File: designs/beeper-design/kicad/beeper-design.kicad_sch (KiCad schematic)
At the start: 0 parts

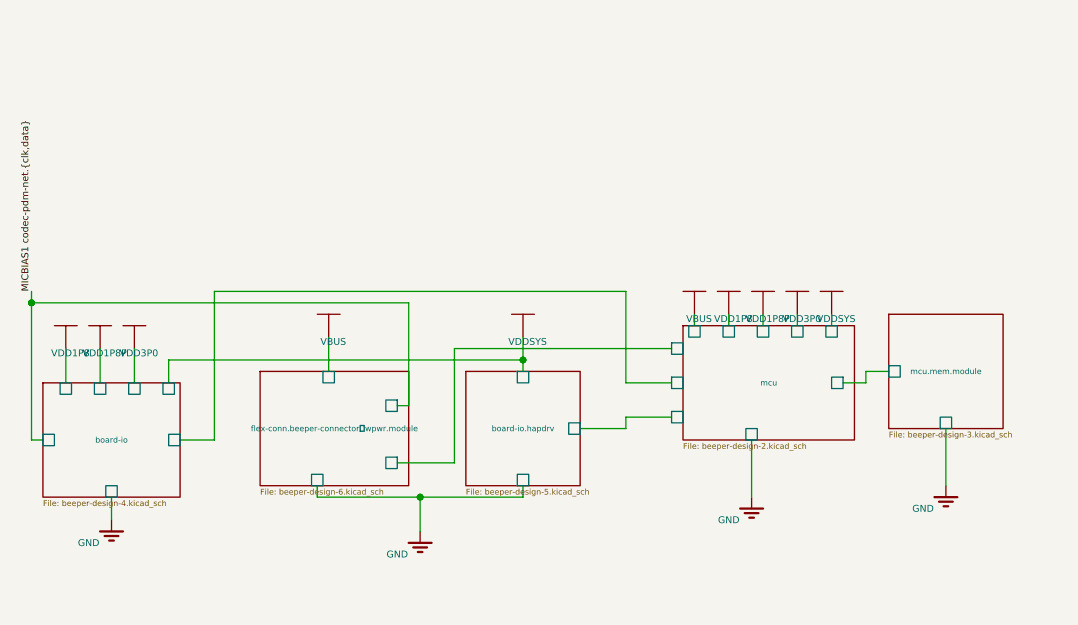
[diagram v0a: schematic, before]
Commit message: new export
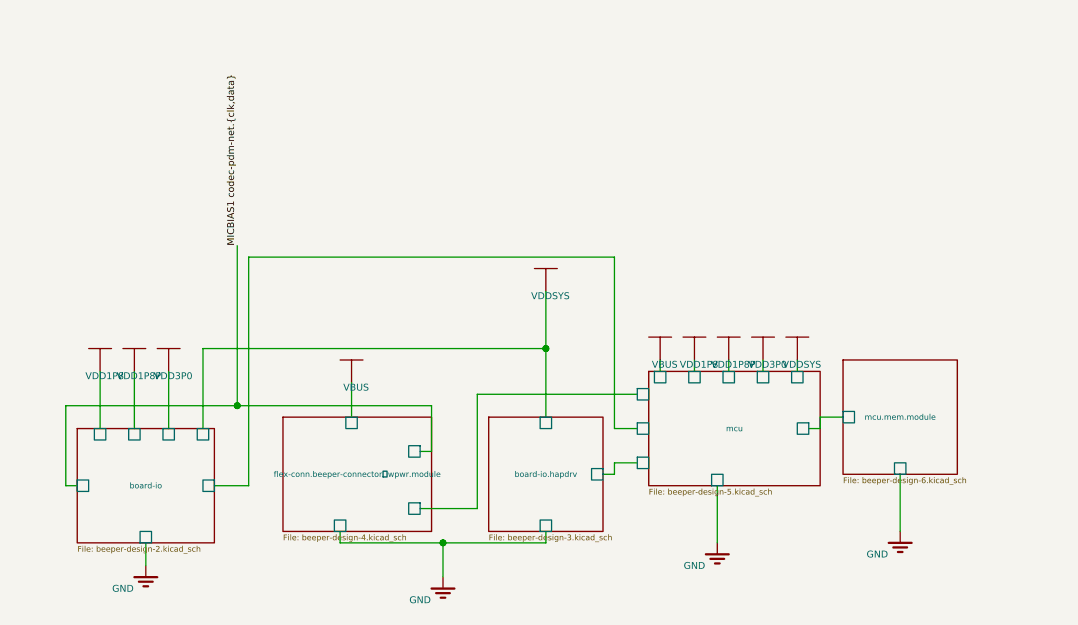
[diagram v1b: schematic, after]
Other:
- sheet board-io: file beeper-design-4.kicad_sch -> beeper-design-2.kicad_sch
- sheet board-io.hapdrv: file beeper-design-5.kicad_sch -> beeper-design-3.kicad_sch
- sheet flex-conn.beeper-connector wpwr.module: file beeper-design-6.kicad_sch -> beeper-design-4.kicad_sch
- sheet mcu: file beeper-design-2.kicad_sch -> beeper-design-5.kicad_sch
- sheet mcu.mem.module: file beeper-design-3.kicad_sch -> beeper-design-6.kicad_sch

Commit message: reasonble export
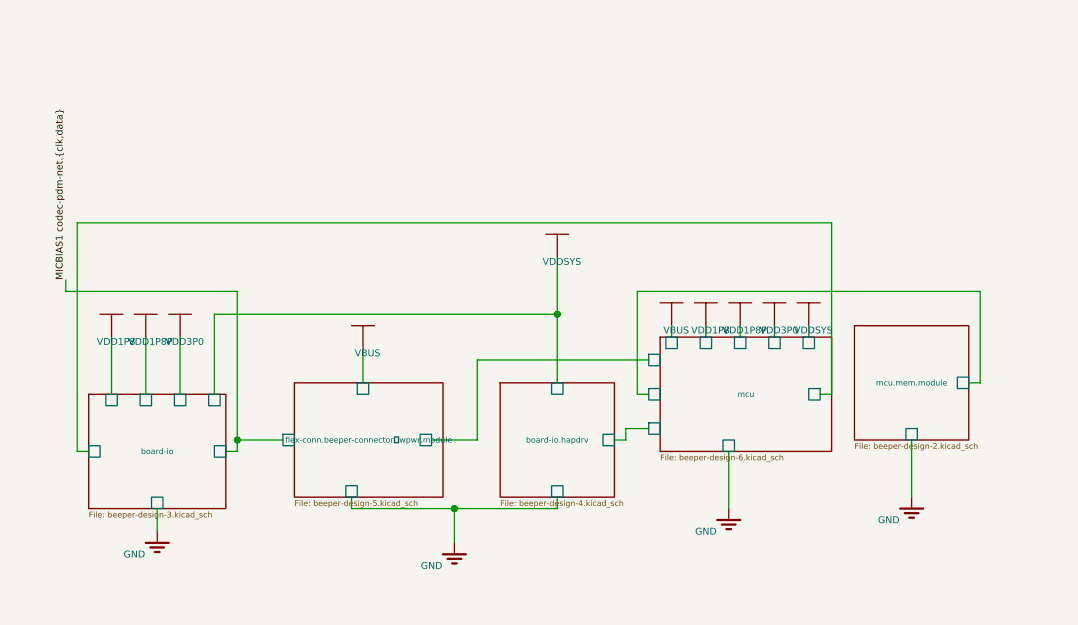
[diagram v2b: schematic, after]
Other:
- sheet board-io: file beeper-design-2.kicad_sch -> beeper-design-3.kicad_sch
- sheet board-io.hapdrv: file beeper-design-3.kicad_sch -> beeper-design-4.kicad_sch
- sheet flex-conn.beeper-connector wpwr.module: file beeper-design-4.kicad_sch -> beeper-design-5.kicad_sch
- sheet mcu: file beeper-design-5.kicad_sch -> beeper-design-6.kicad_sch
- sheet mcu.mem.module: file beeper-design-6.kicad_sch -> beeper-design-2.kicad_sch
